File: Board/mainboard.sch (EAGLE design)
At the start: 14 parts, among them U1 BATTERY-CHARGER-LI-PROT, U2 LF33CDT-TR, U3 TINY13-20PU, U4 ESP12

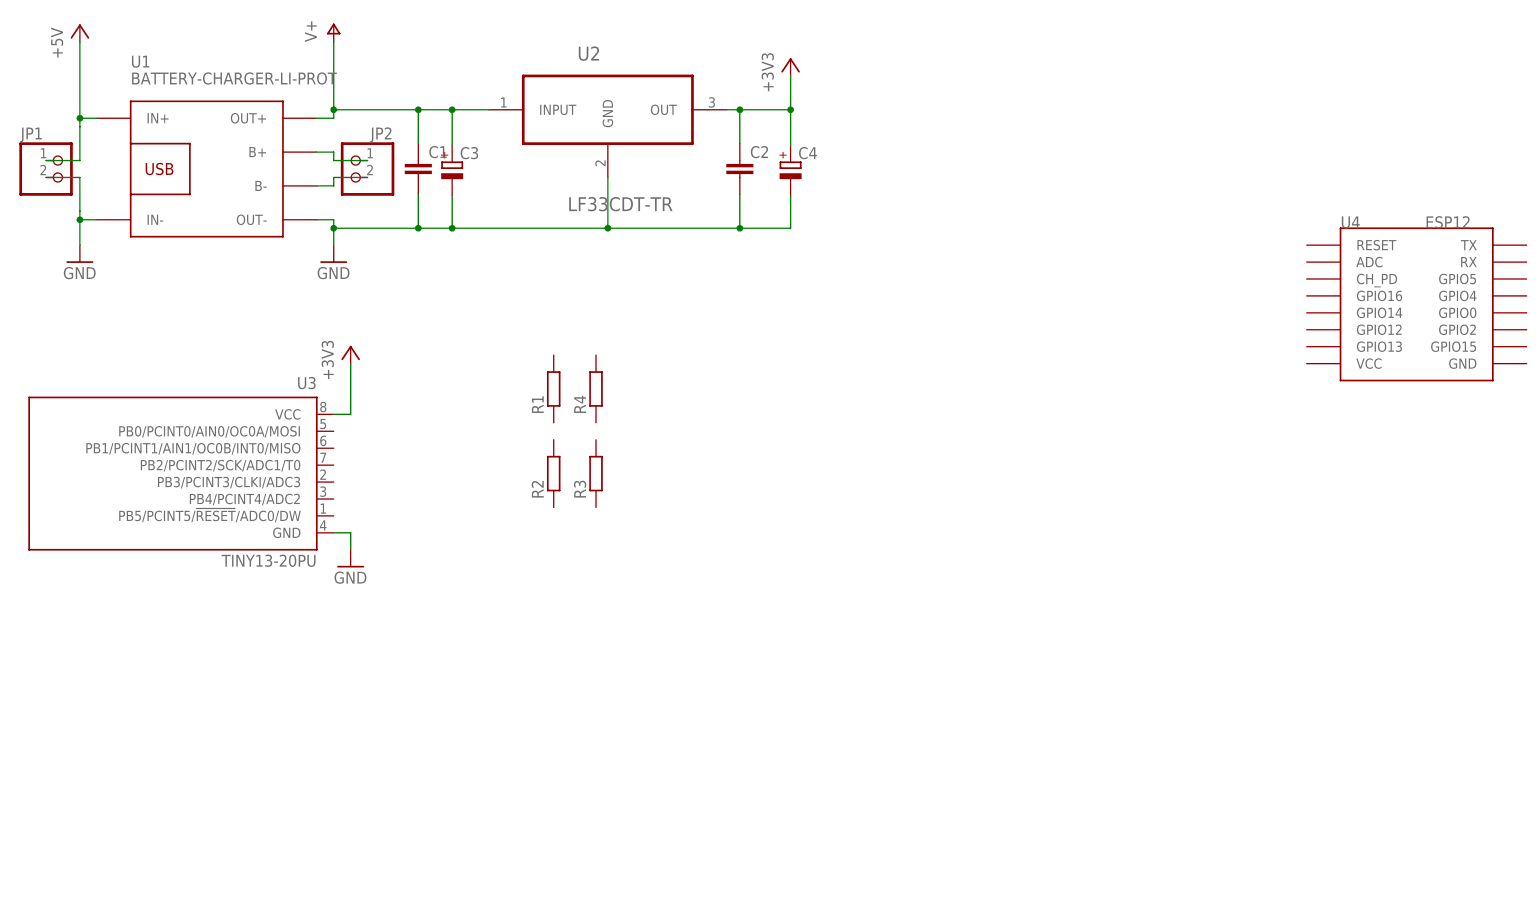
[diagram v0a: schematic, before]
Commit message: Update
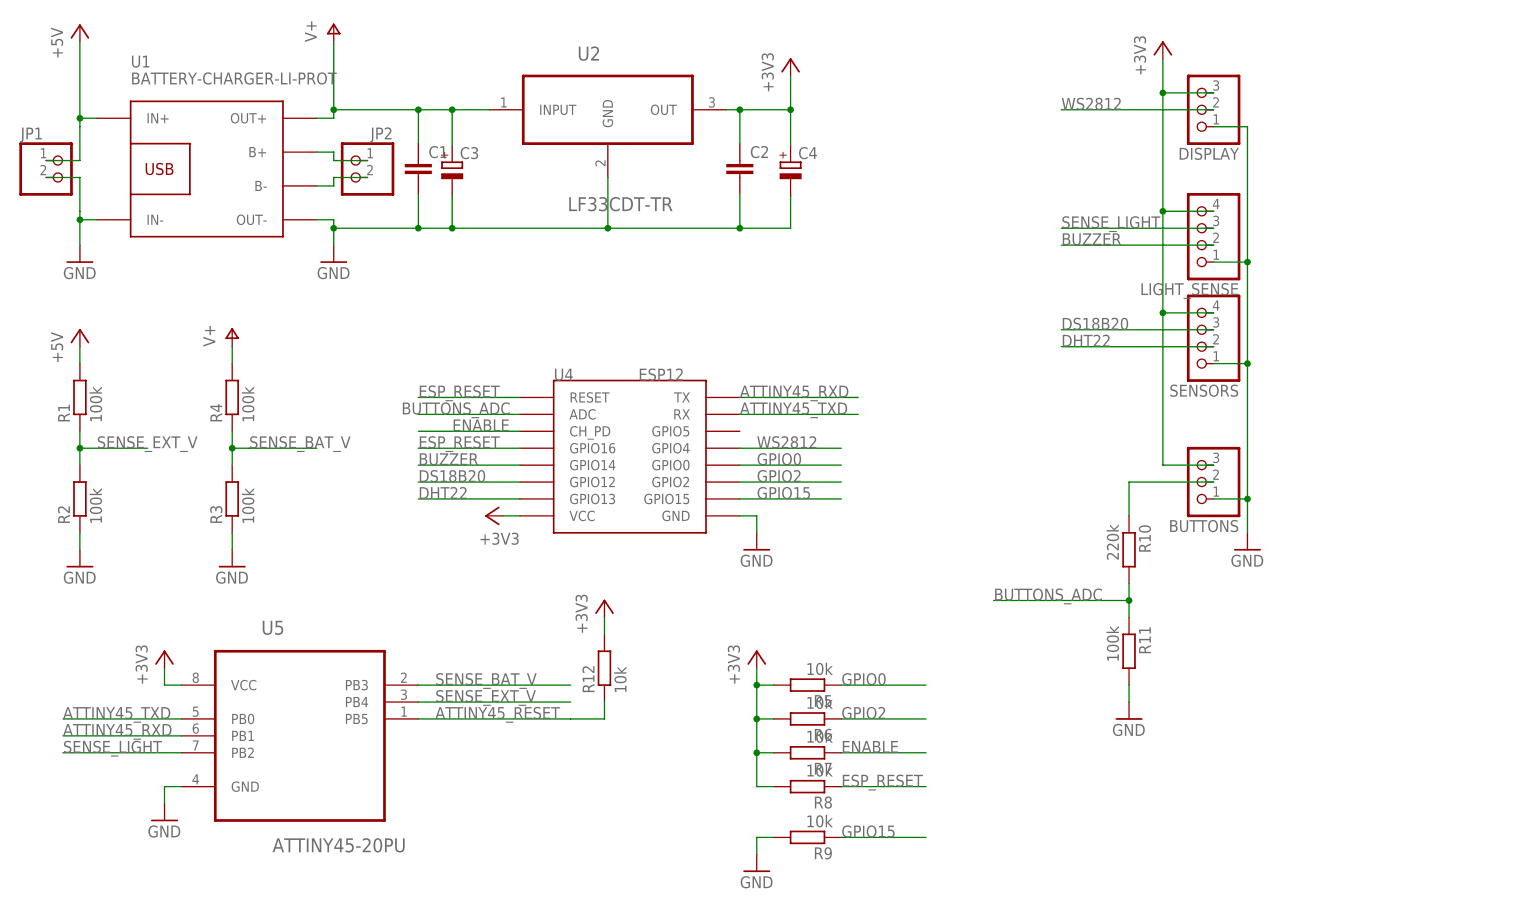
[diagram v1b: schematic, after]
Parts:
- removed U3: TINY13-20PU, atmel:TINY13-20PU
- added BUTTONS, DISPLAY: (no value), pinhead:PINHD-1X3
- added LIGHT_SENSE, SENSORS: (no value), pinhead:PINHD-1X4
- added R10: 220k, rcl:R-EU_R1206
- added R11: 100k, rcl:R-EU_R1206
- added R12, R5, R6, R7, R8, R9: 10k, rcl:R-EU_R1206
- added U5: ATTINY45-20PU, ATTINY45-20PU:ATTINY45-20PU
- R1, R2, R3, R4: value (none) -> 100k
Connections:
- new net ATTINY45_RESET: R12.1, U5.PB5
- new net ATTINY45_RXD: U4.TX, U5.PB1
- new net ATTINY45_TXD: U4.RX, U5.PB0
- new net BUTTONS_ADC: R10.2, R11.1, U4.ADC
- new net BUZZER: LIGHT_SENSE.2, U4.GPIO14
- new net DHT22: SENSORS.2, U4.GPIO13
- new net DS18B20: SENSORS.3, U4.GPIO12
- new net ENABLE: R7.1, U4.CH_PD
- new net ESP_RESET: R8.1, U4.GPIO16, U4.RESET
- new net GPIO0: R5.1, U4.GPIO0
- new net GPIO15: R9.1, U4.GPIO15
- new net GPIO2: R6.1, U4.GPIO2
- new net N$1: BUTTONS.2, R10.1
- new net SENSE_BAT_V: R3.2, R4.1, U5.PB3
- new net SENSE_EXT_V: R1.1, R2.2, U5.PB4
- new net SENSE_LIGHT: LIGHT_SENSE.3, U5.PB2
- new net WS2812: DISPLAY.2, U4.GPIO4
- net +3V3: now also BUTTONS.3, DISPLAY.3, LIGHT_SENSE.4, R12.2, R5.2, R6.2, R7.2, R8.2, SENSORS.4, U4.VCC, U5.VCC; no longer U3.VCC
- net +5V: now also R1.2
- net GND: now also BUTTONS.1, DISPLAY.1, LIGHT_SENSE.1, R11.2, R2.1, R3.1, R9.2, SENSORS.1, U4.GND, U5.GND; no longer U3.GND
- net V+: now also R4.2
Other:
- moved on the sheet: R1, R2, R3, R4, U4
